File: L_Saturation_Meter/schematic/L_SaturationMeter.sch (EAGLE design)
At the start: 40 parts, among them IC1 LM317, IC4 LM358, T1 IRF830, T2 BC847, T3 BC857, X2 POWER_12V, X3 L_TEST, X4 I_SENSE

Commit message: Fix CE packages pads naming, to avoid inconsistance after package change
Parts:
- C2: device __MyCommonLib1:CE10MM -> __MyCommonLib1:CE8.2MM
- C4: device __MyCommonLib1:CE6.3MM -> __MyCommonLib1:CE5.2MM
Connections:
- net +VCC: now also C4.PLUS; no longer C4.+
- net GND: now also C100.MINUS, C2.MINUS, C4.MINUS, C8.MINUS; no longer C100.-, C2.-, C4.-, C8.-
- net N$11: now also C2.PLUS; no longer C2.+
- net N$6: now also C104.MINUS; no longer C104.-
- net N$9: now also C100.PLUS, C104.PLUS, C8.PLUS; no longer C100.+, C104.+, C8.+

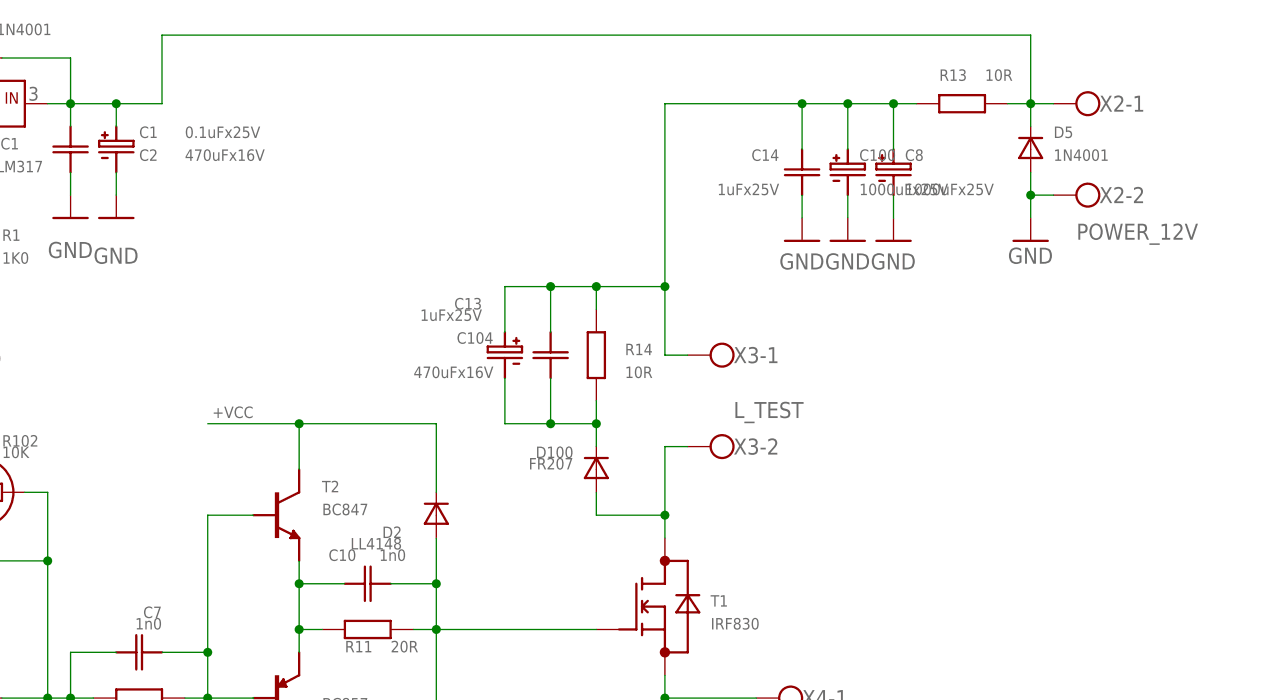
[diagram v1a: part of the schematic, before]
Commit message: Start routing
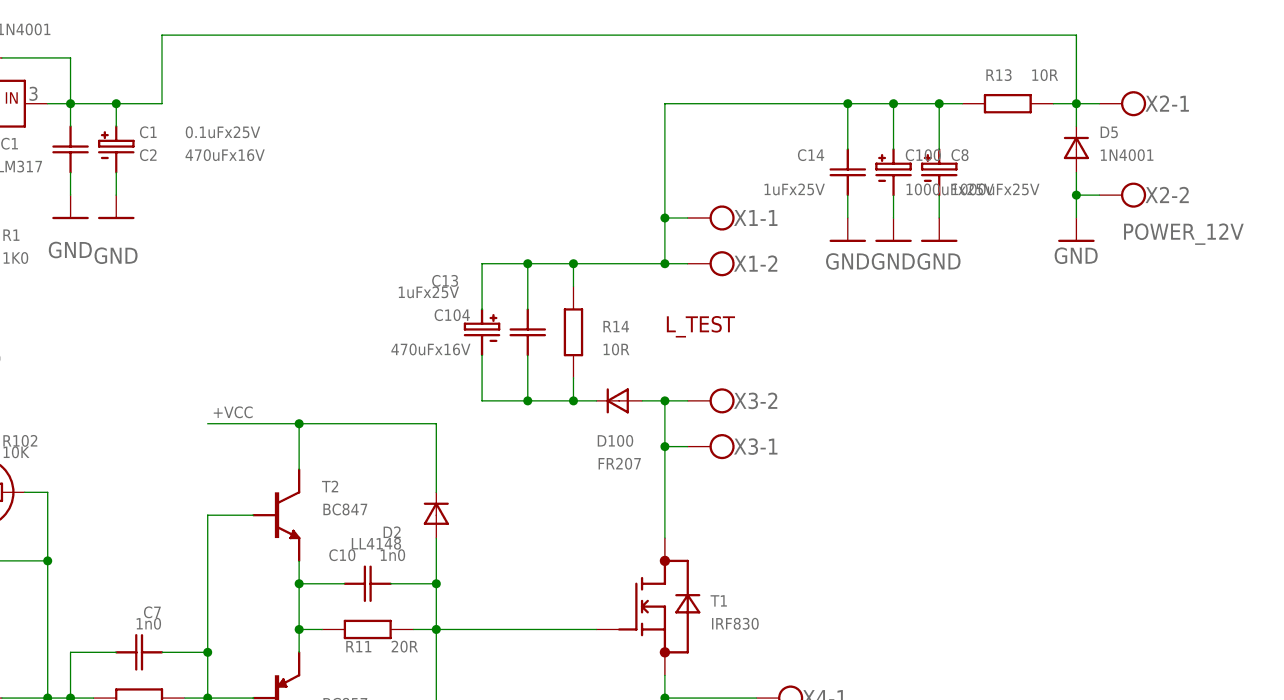
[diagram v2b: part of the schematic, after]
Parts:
- added X1: (no value), con-wago-500:W237-102
- D5: device __MyCommonLib1:1N4001DO-41_10MM -> __MyCommonLib1:1N4001DO-41_5MM
- R12: device __MyCommonLib1:R2.0W -> __MyCommonLib1:R1.0W_VERT
- R14: device __MyCommonLib1:R1.0W -> __MyCommonLib1:R1.0W_VERT
- X3: value L_TEST -> (none)
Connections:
- net N$10: now also X3-1.KL
- net N$9: now also X1-1.KL, X1-2.KL; no longer X3-1.KL
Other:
- note added: "L_TEST"
- moved on the sheet: C100, C104, C13, C14, C8, D100, D5, R13, R14, X2-1, X2-2, X3-1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

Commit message: L saturation metter routed
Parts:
- X1: value (none) -> L_TEST_START
- X3: value (none) -> L_TEST_END
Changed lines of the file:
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@@
 <part name="R13" library="__MyCommonLib1" deviceset="R" device="2.0W" value="10R"/>
 <part name="X2" library="con-wago-500" deviceset="W237-102" device="" value="POWER_12V"/>
-<part name="X3" library="con-wago-500" deviceset="W237-102" device=""/>
+<part name="X3" library="con-wago-500" deviceset="W237-102" device="" value="L_TEST_END"/>
 <part name="X4" library="con-wago-500" deviceset="W237-102" device="" value="I_SENSE"/>
 <part name="GND4" library="supply1" deviceset="GND" device=""/>
@@
 <part name="C8" library="__MyCommonLib1" deviceset="CE" device="10MM" value="1000uFx25V"/>
 <part name="C104" library="__MyCommonLib1" deviceset="CE" device="8.2MM" value="470uFx16V"/>
-<part name="X1" library="con-wago-500" deviceset="W237-102" device="">
+<part name="X1" library="con-wago-500" deviceset="W237-102" device="" value="L_TEST_START">
 <attribute name="MF" value=""/>
 <attribute name="MPN" value="237-102"/>
@@
 </instance>
 <instance part="X3" gate="-2" x="200.66" y="129.54" smashed="yes" rot="MR0">
-<attribute name="VALUE" x="203.2" y="126.873" size="1.778" layer="96" rot="MR180"/>
 <attribute name="NAME" x="200.66" y="130.429" size="1.778" layer="95" rot="MR180"/>
 </instance>
@@
 <attribute name="NAME" x="200.66" y="150.749" size="1.778" layer="95" rot="MR180"/>
 </instance>
-<instance part="X1" gate="-2" x="200.66" y="144.78" rot="MR0"/>
+<instance part="X1" gate="-2" x="200.66" y="144.78" smashed="yes" rot="MR0">
+<attribute name="NAME" x="200.66" y="145.669" size="1.778" layer="95" rot="MR180"/>
+</instance>
 </instances>
 <busses>
